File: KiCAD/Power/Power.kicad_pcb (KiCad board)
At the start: 4 copper layers, 30 x 100 mm, 23 parts, among them J1 Barrel_Jack_Switch_MountingPin, J2 Conn_01x03_Pin, U1 LM317 TO-220, U2 LM337 TO-220, U3 LM336Z-2.5v

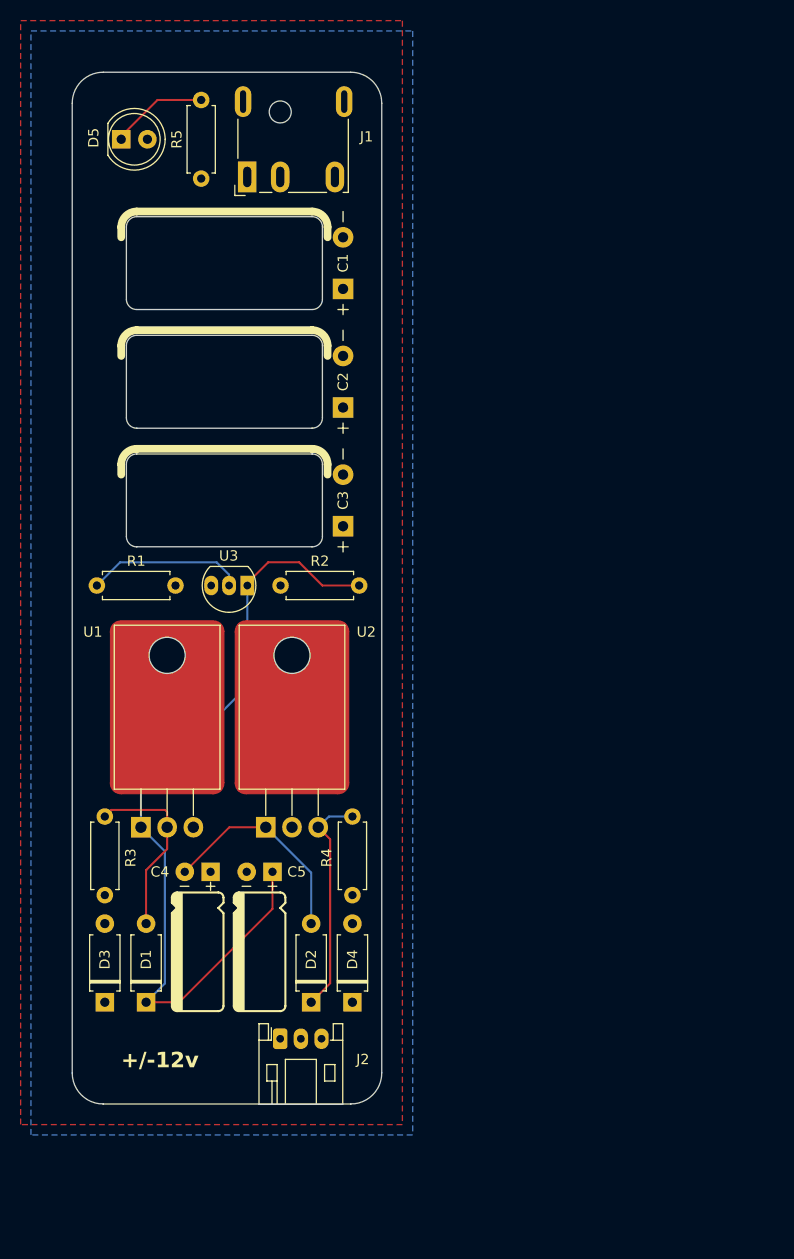
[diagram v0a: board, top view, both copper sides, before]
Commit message: Mixer PCB - Gerbers
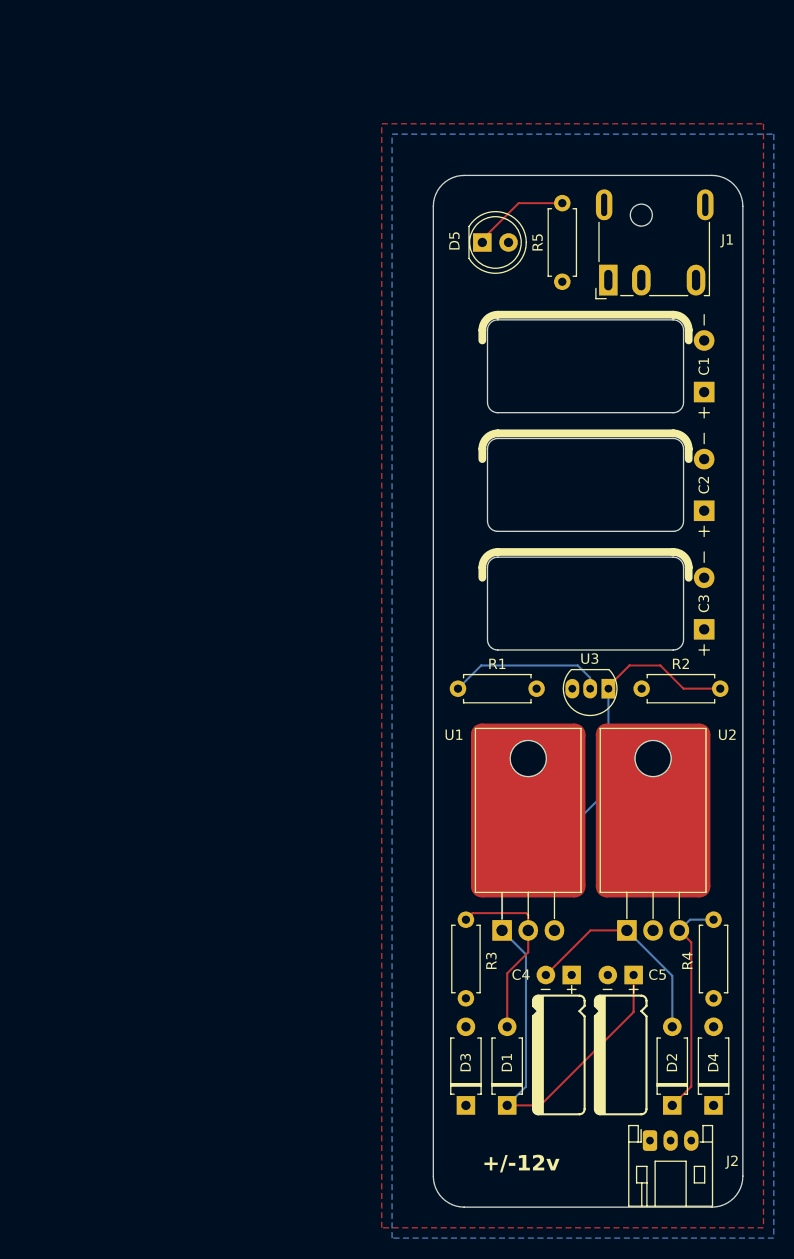
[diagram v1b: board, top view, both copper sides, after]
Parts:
- added REF**: Untitled, HackSynth:Module 30x100mm, F.Cu at (150.0, 100.0)
- moved J2 37.2 mm to (156.0, 143.6)
- moved J1 36.4 mm to (152.0, 60.1)
- moved C1 36.4 mm to (161.2, 71.0)
- moved C2 36.4 mm to (161.2, 82.5)
- moved C3 36.4 mm to (161.2, 94.0)
- moved C4 36.4 mm to (147.2, 127.5)
- moved C5 36.4 mm to (153.2, 127.5)
- moved D1 36.4 mm to (142.2, 140.1)
- moved D2 36.4 mm to (158.2, 140.1)
- moved D3 36.4 mm to (138.2, 140.1)
- moved D4 36.4 mm to (162.2, 140.1)
- moved D5 36.4 mm to (139.8, 56.5)
- moved R2 36.4 mm to (155.2, 99.8)
- moved R3 36.4 mm to (138.2, 129.8)
- moved R4 36.4 mm to (162.2, 122.1)
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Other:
- board text added: "POWER v1-1 - PancakeLegend 2025"
- board text removed: "POWER v1-0 - PancakeLegend 2025"
